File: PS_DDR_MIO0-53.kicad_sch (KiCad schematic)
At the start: 1 part, among them U13 XCZU15EG-2FFVB1156E

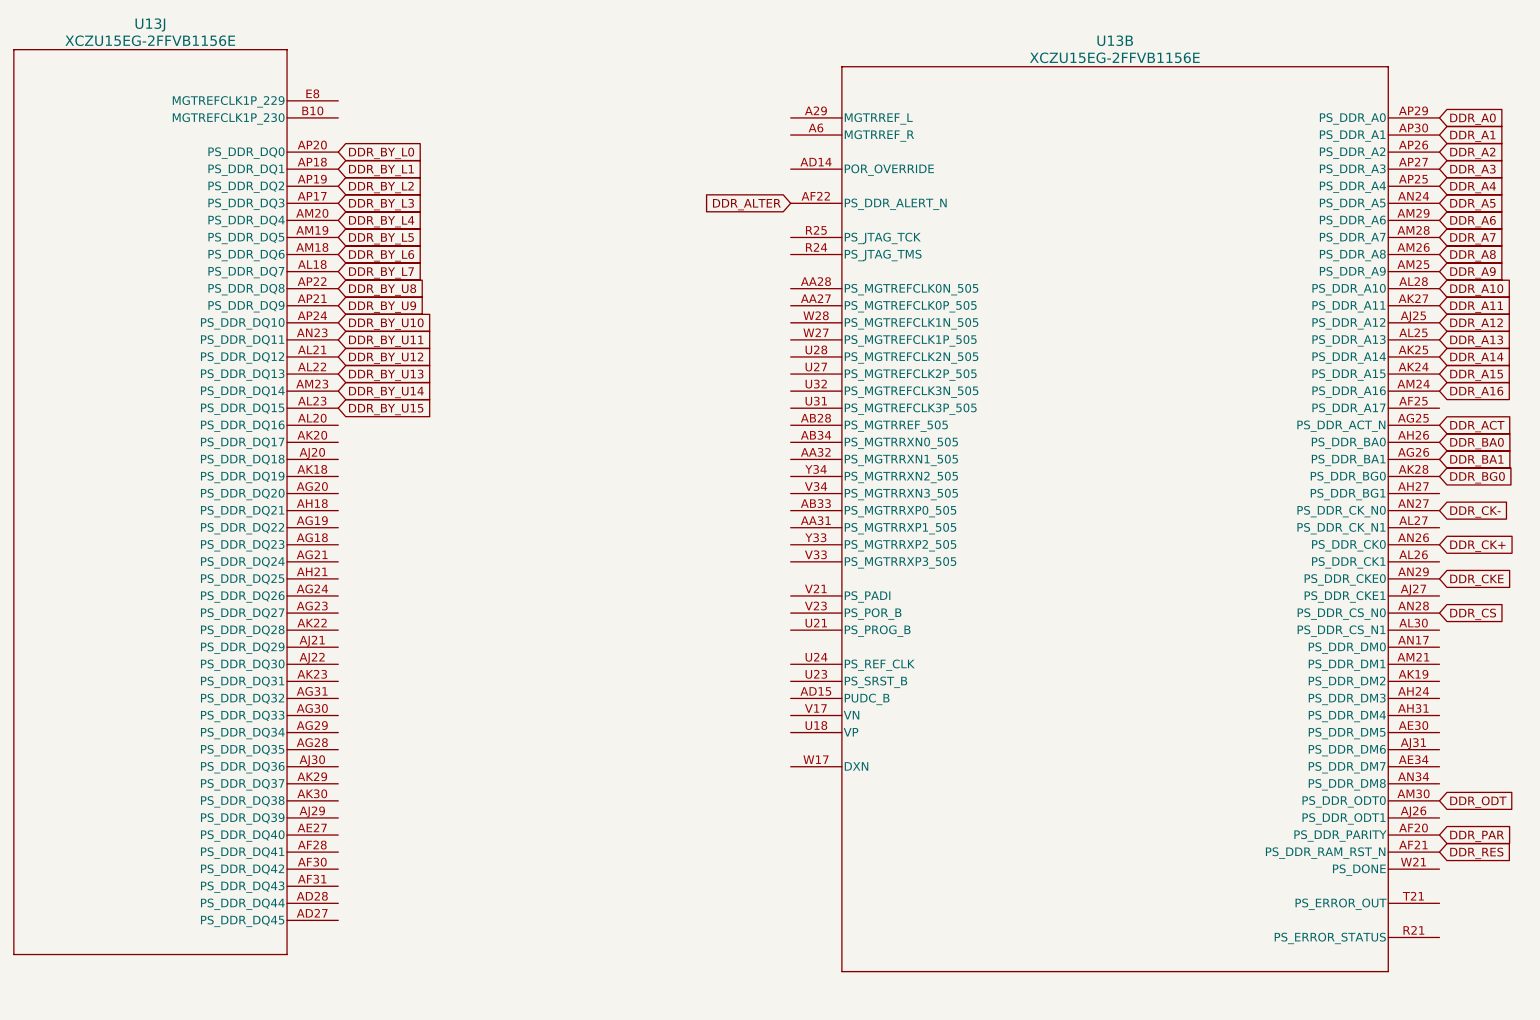
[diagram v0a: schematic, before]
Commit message: Stuff
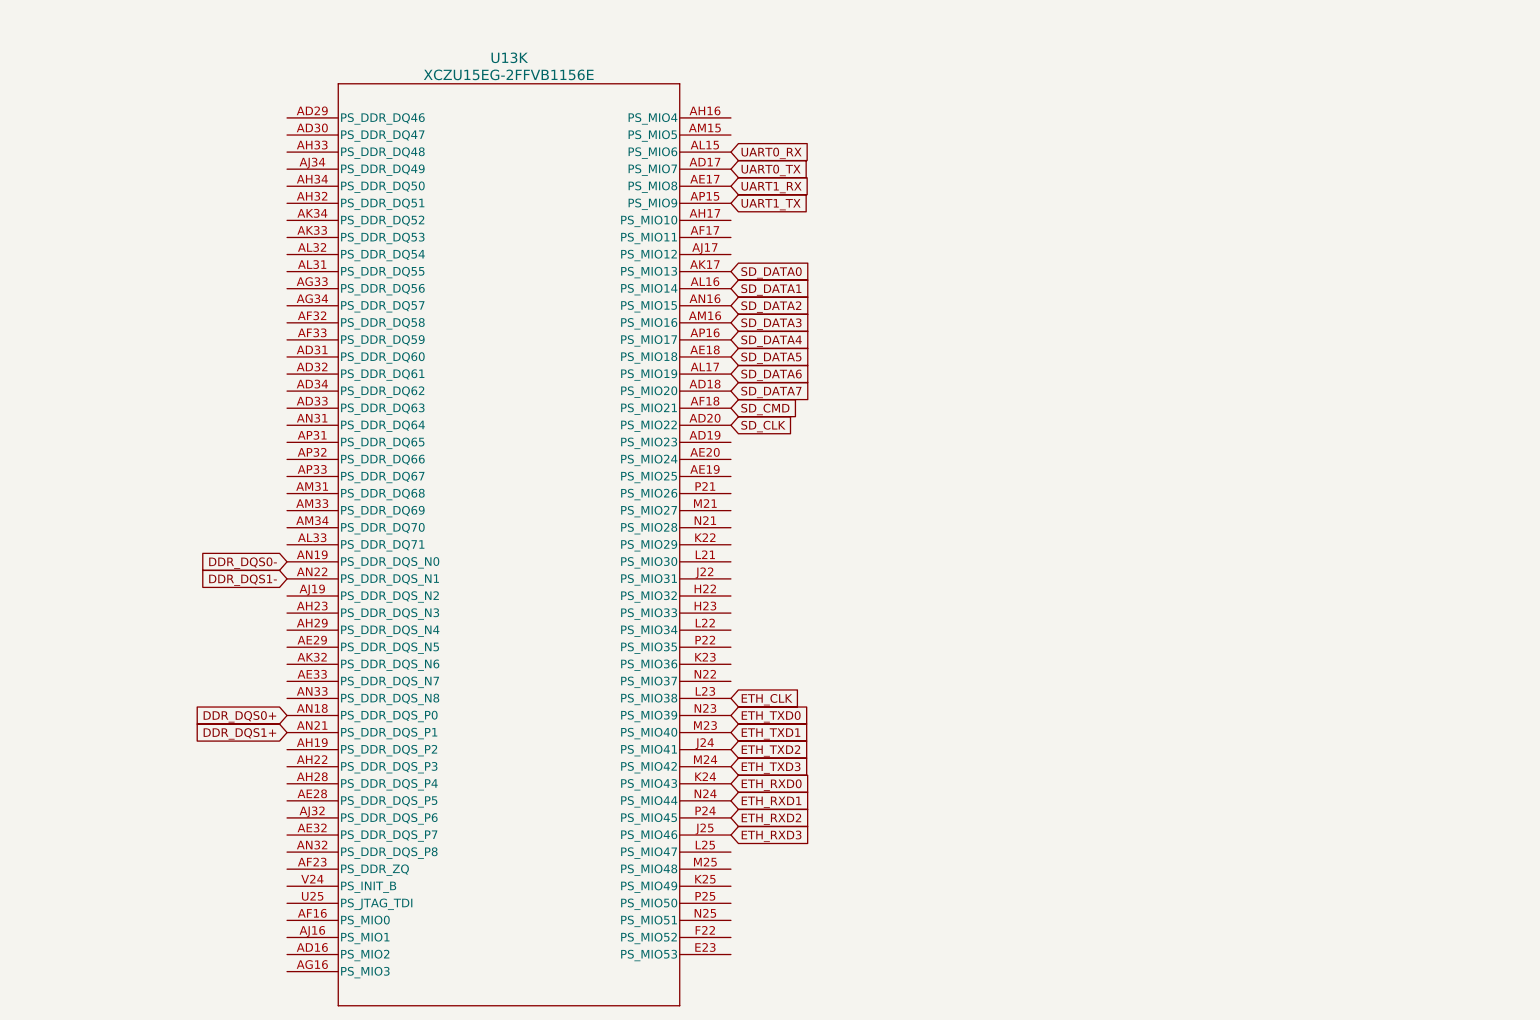
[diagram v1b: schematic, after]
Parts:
- removed U13: XCZU15EG-2FFVB1156E, lib:FFVB1156_XIL-L, symbol XCZU15EG:XCZU15EG-2FFVB1156E
- added U13: XCZU15EG-2FFVB1156E, lib:FFVB1156_XIL-L, symbol XCZU15EG:XCZU15EG-2FFVB1156E
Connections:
- new net DDR_DQS0+: U13.AN18 (PS_DDR_DQS_P0)
- new net DDR_DQS0-: U13.AN19 (PS_DDR_DQS_N0)
- new net DDR_DQS1+: U13.AN21 (PS_DDR_DQS_P1)
- new net DDR_DQS1-: U13.AN22 (PS_DDR_DQS_N1)
- new net ETH_CLK: U13.L23 (PS_MIO38)
- new net ETH_RXD0: U13.K24 (PS_MIO43)
- new net ETH_RXD1: U13.N24 (PS_MIO44)
- new net ETH_RXD2: U13.P24 (PS_MIO45)
- new net ETH_RXD3: U13.J25 (PS_MIO46)
- new net ETH_TXD0: U13.N23 (PS_MIO39)
- new net ETH_TXD1: U13.M23 (PS_MIO40)
- new net ETH_TXD2: U13.J24 (PS_MIO41)
- new net ETH_TXD3: U13.M24 (PS_MIO42)
- new net SD_CLK: U13.AD20 (PS_MIO22)
- new net SD_CMD: U13.AF18 (PS_MIO21)
- new net SD_DATA0: U13.AK17 (PS_MIO13)
- new net SD_DATA1: U13.AL16 (PS_MIO14)
- new net SD_DATA2: U13.AN16 (PS_MIO15)
- new net SD_DATA3: U13.AM16 (PS_MIO16)
- new net SD_DATA4: U13.AP16 (PS_MIO17)
- new net SD_DATA5: U13.AE18 (PS_MIO18)
- new net SD_DATA6: U13.AL17 (PS_MIO19)
- new net SD_DATA7: U13.AD18 (PS_MIO20)
- new net UART0_RX: U13.AL15 (PS_MIO6)
- new net UART0_TX: U13.AD17 (PS_MIO7)
- new net UART1_RX: U13.AE17 (PS_MIO8)
- new net UART1_TX: U13.AP15 (PS_MIO9)
